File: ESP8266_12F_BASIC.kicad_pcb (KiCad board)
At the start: 2 copper layers, 64.7 x 63.5 mm, 40 parts, among them J1 Conn_01x02_Male, J2 Conn_01x04_Male, J3 Conn_01x05_Female, Q1 BC547, U1 ESP-12F, U2 AP1117-33

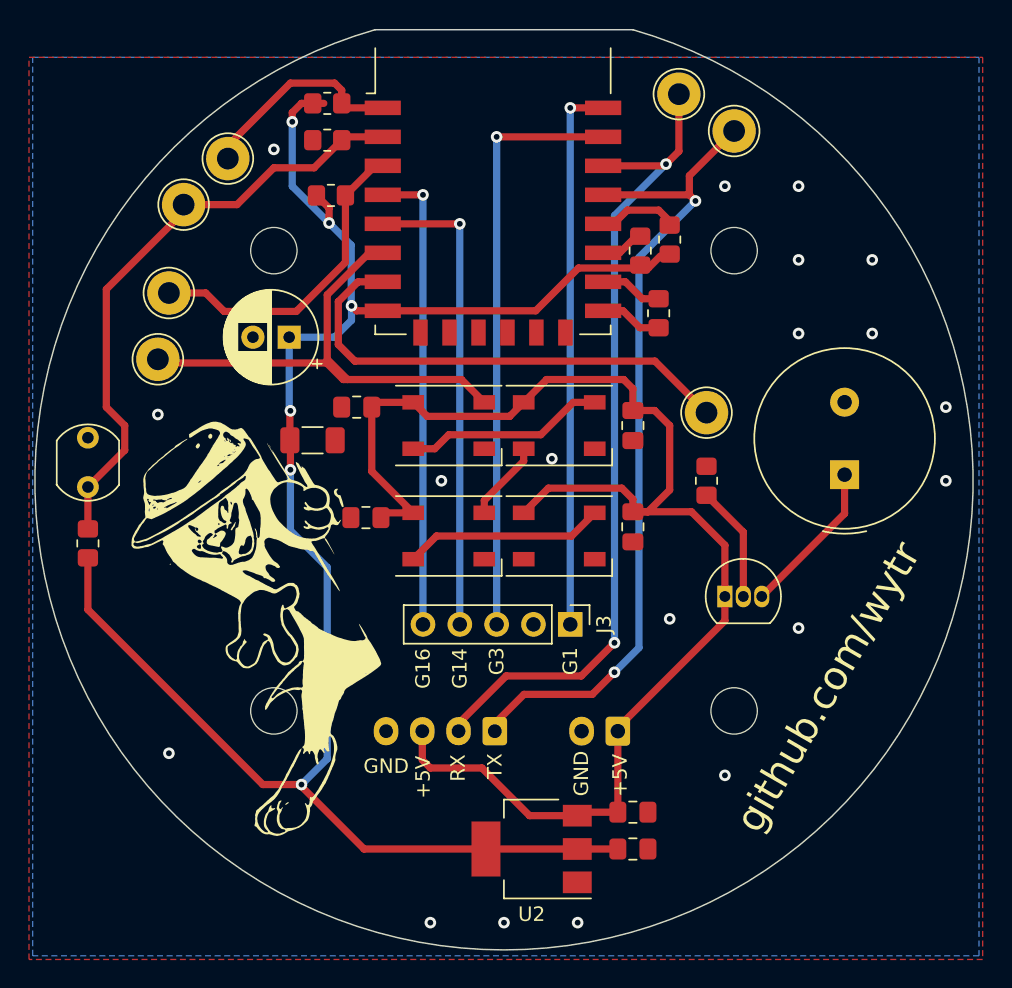
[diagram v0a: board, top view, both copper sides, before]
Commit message: weird shit
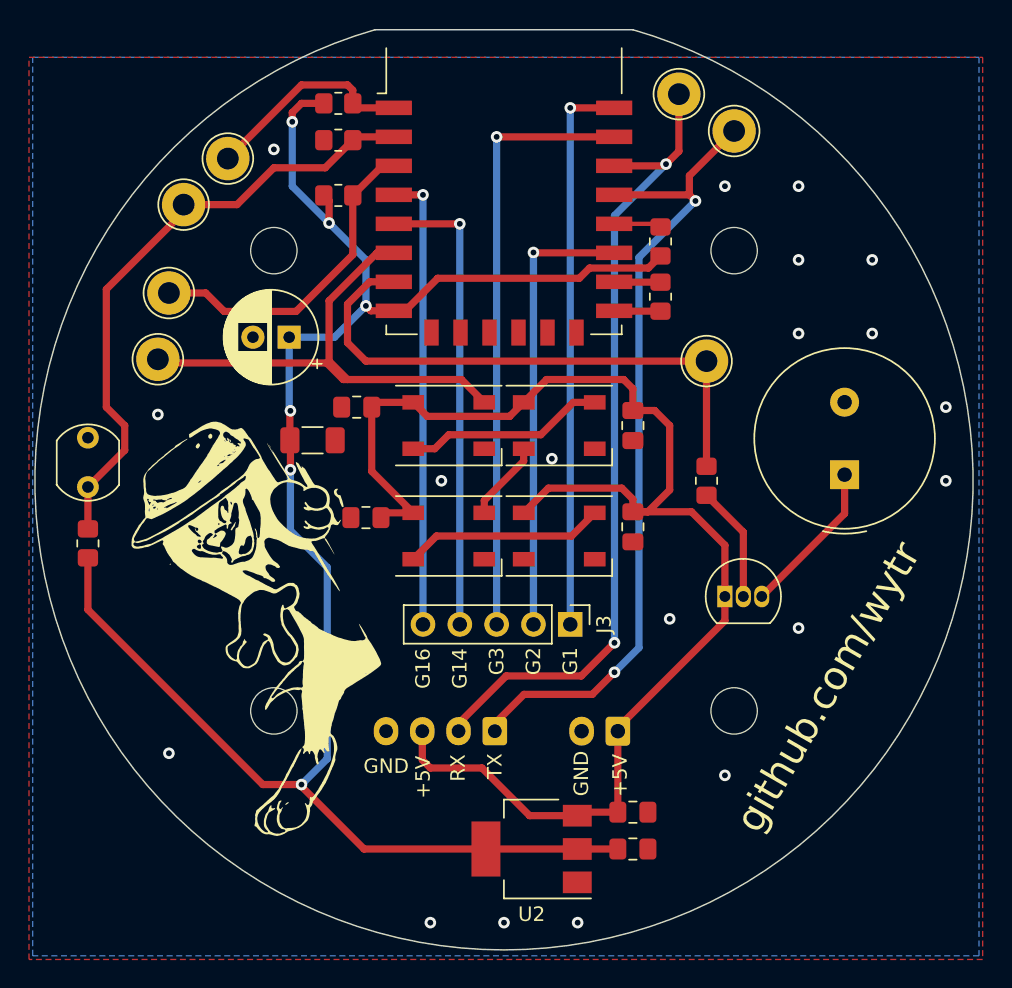
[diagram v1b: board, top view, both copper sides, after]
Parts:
- removed R8: 10k, Resistor_SMD:R_0805_2012Metric_Pad1.20x1.40mm_HandSolder
- moved TP3 3.56 mm to (166.4, 93.3)
- moved R6 1.15 mm to (163.2, 88.9)
- moved R2 0.76 mm to (141.0, 78.1)
- moved R3 0.76 mm to (141.0, 75.6)
- moved U1 0.76 mm to (152.4, 79.4)
- moved R5 0.65 mm to (163.2, 85.1)
- moved R4 0.51 mm to (141.0, 81.9)
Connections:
- J3 pad 2: unconnected-(J3-Pad2) -> GPIO2
- U1 pad 17: Net-(R8-Pad2) -> GPIO2
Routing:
- net GPIO2: track 0.00 -> 31.0 mm, vias 0 -> 1
- net BUZZ: track 35.6 -> 39.0 mm
- net Net-(R8-Pad2): track 3.04 -> 0.00 mm
- net Net-(R5-Pad2): track 5.57 -> 3.28 mm
- net GND: track 4.35 -> 3.21 mm
- net Net-(R6-Pad2): track 4.31 -> 3.21 mm
- net ESP_ADC: track 41.5 -> 42.3 mm
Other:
- board text added: "G2"
